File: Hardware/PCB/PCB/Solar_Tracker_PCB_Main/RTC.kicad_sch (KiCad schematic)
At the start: 1 part, among them IC4 PCF2131TFY

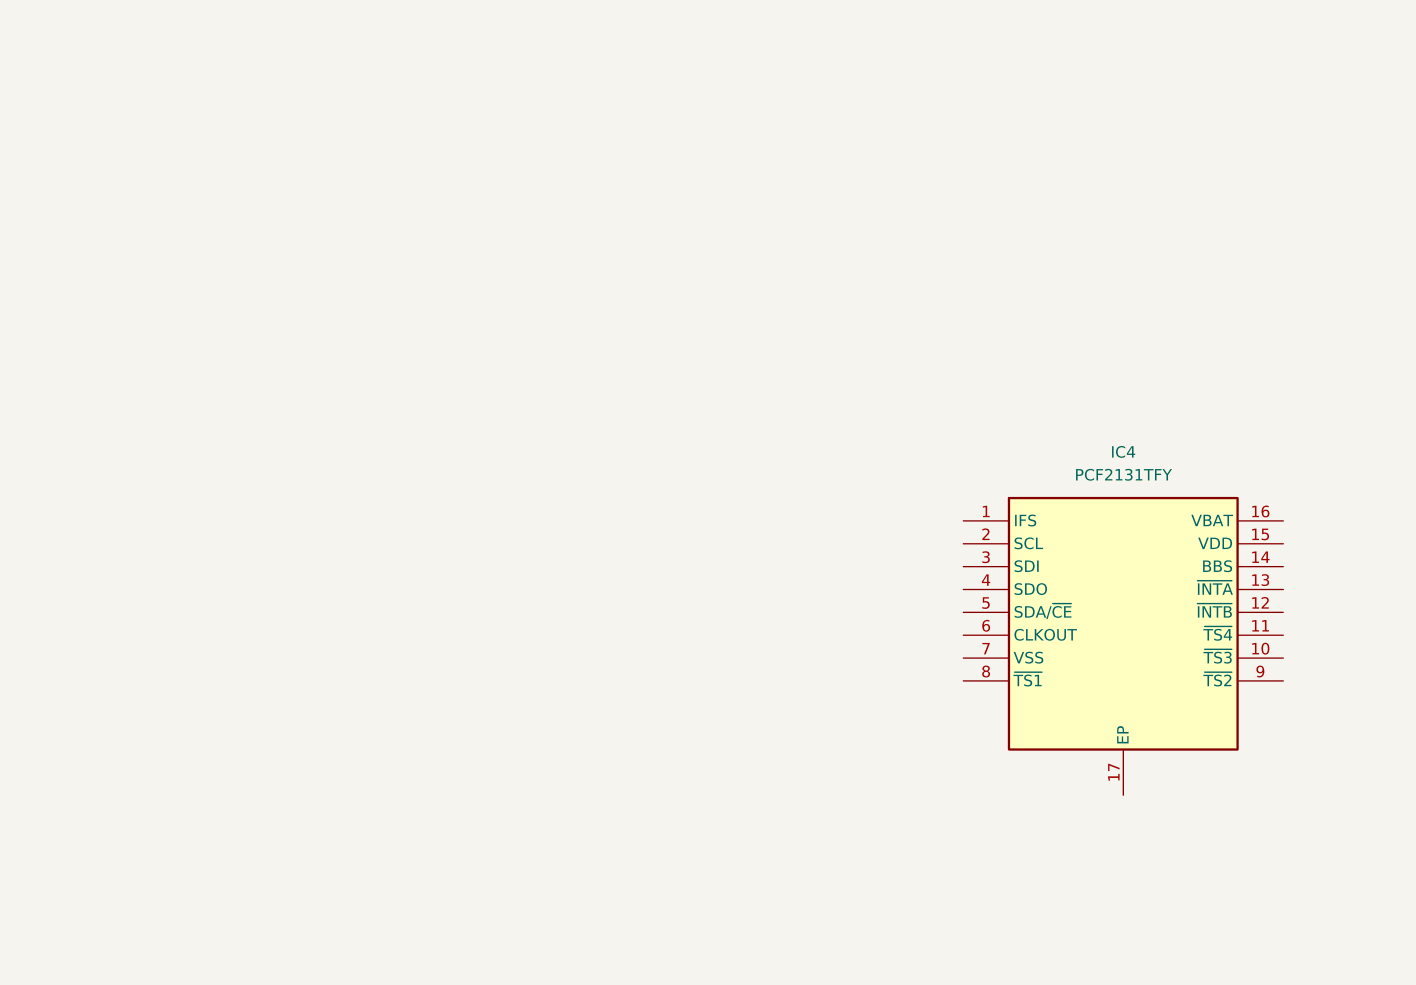
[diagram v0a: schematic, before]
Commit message: Actualizacion PCB Principal
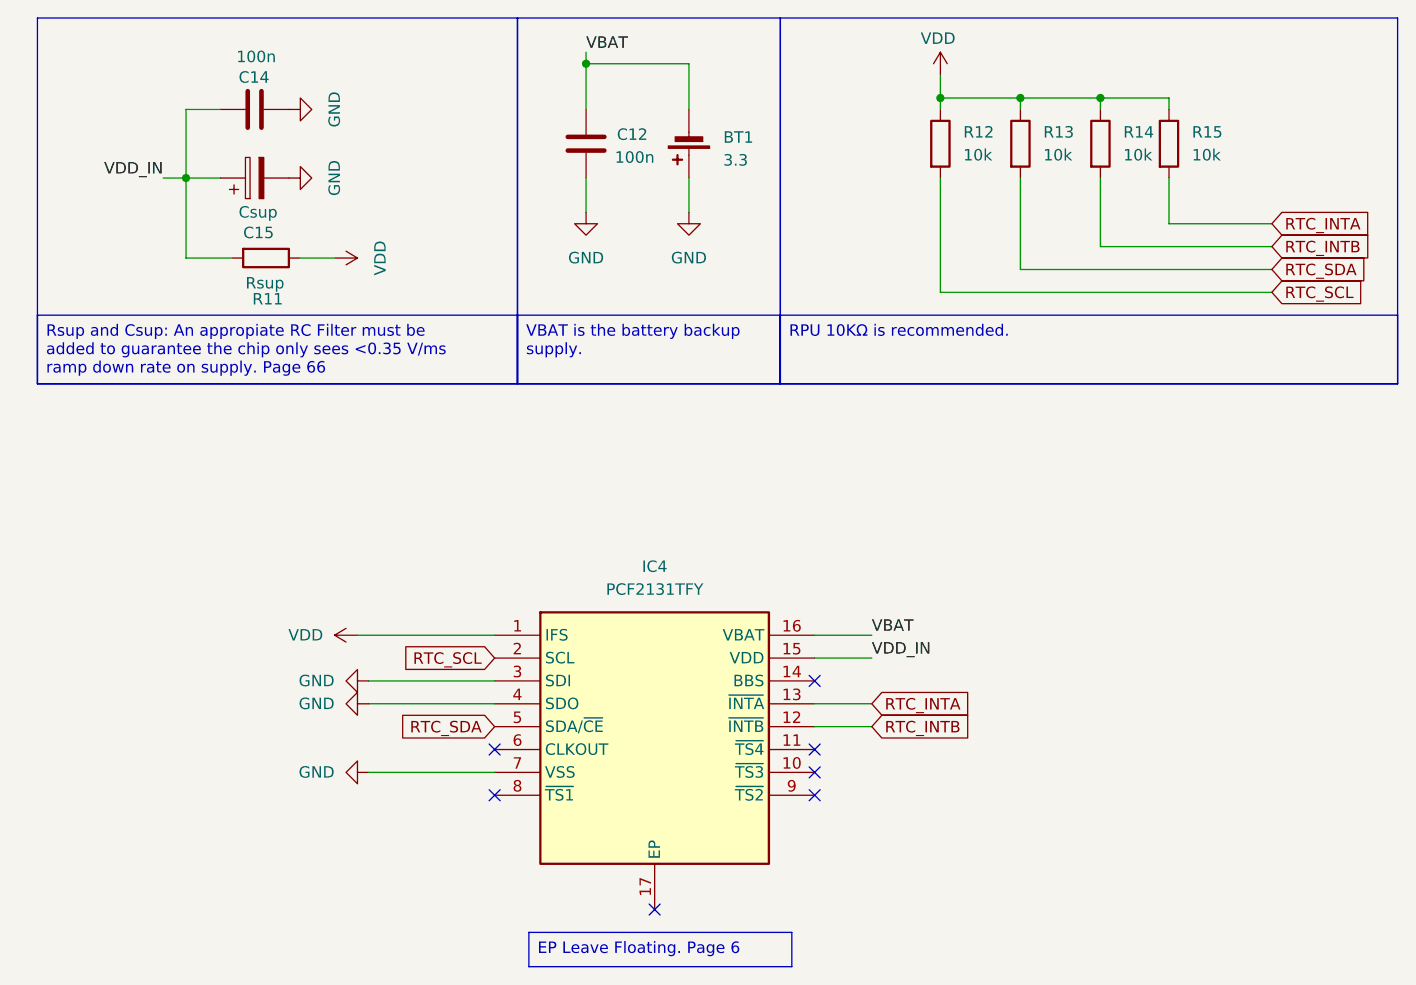
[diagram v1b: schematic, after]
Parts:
- added BT1: 3.3, symbol Device:Battery_Cell
- added C12, C14: 100n, symbol Device:C
- added C15: Csup, symbol Device:C_Polarized
- added R11: Rsup, symbol Device:R
- added R12, R13, R14, R15: 10k, symbol Device:R
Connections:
- net VDD: now reaches IC4.1 (IFS)
- net VDD: now also R11.1, R12.1, R13.1, R14.1, R15.1
- net RTC_INTB: now reaches IC4.12 (~{INTB})
- net RTC_INTB: now also R14.2
- net RTC_INTA: now reaches IC4.13 (~{INTA})
- net RTC_INTA: now also R15.2
- net VDD_IN: now reaches IC4.15 (VDD)
- net VDD_IN: now also C14.2, C15.1, R11.2
- net VBAT: now reaches IC4.16 (VBAT)
- net VBAT: now also BT1.2 (-), C12.2
- net RTC_SCL: now reaches IC4.2 (SCL)
- net RTC_SCL: now also R12.2
- net GND: now reaches IC4.3 (SDI)
- net GND: now also IC4.4 (SDO), IC4.7 (VSS), BT1.1 (+), C12.1, C14.1, C15.2
- net RTC_SDA: now reaches IC4.5 (SDA/~{CE})
- net RTC_SDA: now also R13.2
- no-connect marks 0 -> 7
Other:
- moved on the sheet: IC4

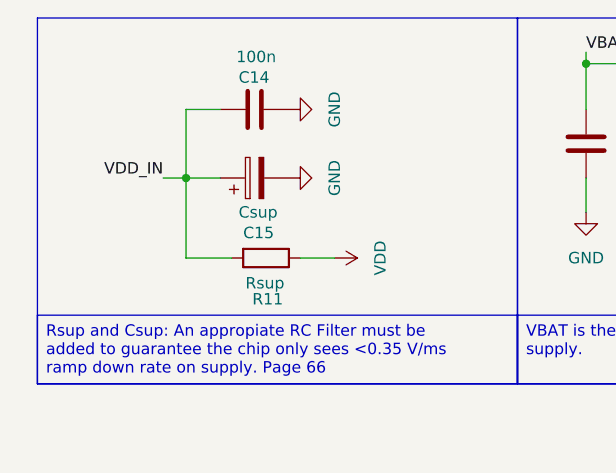
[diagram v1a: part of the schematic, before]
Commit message: actualizacion pcb principal
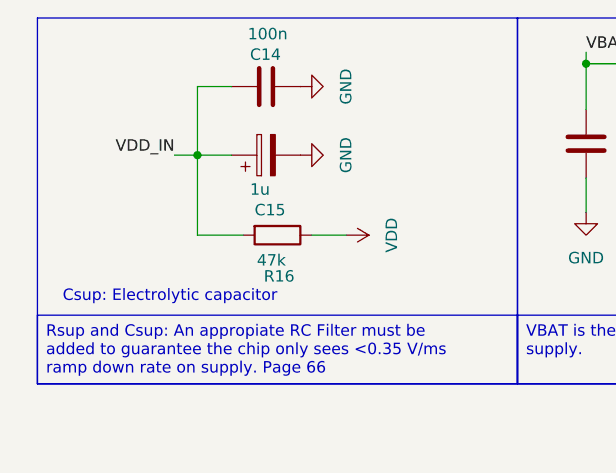
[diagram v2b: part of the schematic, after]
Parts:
- C15: value Csup -> 1u
- R16: renamed from R11; value Rsup -> 47k
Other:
- note added: "Csup: Electrolytic capacitor"
- moved on the sheet: C14, C15, R16
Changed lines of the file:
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@@
+		)
+	)
+	(text "Csup: Electrolytic capacitor"
+		(exclude_from_sim no)
+		(at 27.432 43.688 0)
+		(effects
+			(font
+				(size 1.27 1.27)
+			)
 		)
 	)
@@
 	)
 	(junction
-		(at 29.21 30.48)
+		(at 30.48 27.94)
 		(diameter 0)
 		(color 0 0 0 0)
@@
 	(wire
 		(pts
-			(xy 33.02 22.86) (xy 29.21 22.86)
-		)
-		(stroke
-			(width 0)
-			(type default)
-		)
-	)
-	(wire
-		(pts
-			(xy 34.29 39.37) (xy 29.21 39.37)
-		)
-		(stroke
-			(width 0)
-			(type default)
-		)
-	)
-	(wire
-		(pts
-			(xy 33.02 30.48) (xy 29.21 30.48)
+			(xy 34.29 20.32) (xy 30.48 20.32)
+		)
+		(stroke
+			(width 0)
+			(type default)
+		)
+	)
+	(wire
+		(pts
+			(xy 35.56 36.83) (xy 30.48 36.83)
+		)
+		(stroke
+			(width 0)
+			(type default)
+		)
+	)
+	(wire
+		(pts
+			(xy 34.29 27.94) (xy 30.48 27.94)
 		)
 		(stroke
@@
 	(wire
 		(pts
-			(xy 26.67 30.48) (xy 29.21 30.48)
+			(xy 27.94 27.94) (xy 30.48 27.94)
 		)
 		(stroke
@@
 	(wire
 		(pts
-			(xy 29.21 39.37) (xy 29.21 30.48)
+			(xy 30.48 36.83) (xy 30.48 27.94)
 		)
 		(stroke
@@
 	(wire
 		(pts
-			(xy 29.21 22.86) (xy 29.21 30.48)
+			(xy 30.48 20.32) (xy 30.48 27.94)
 		)
 		(stroke
@@
 	(wire
 		(pts
-			(xy 41.91 39.37) (xy 45.72 39.37)
+			(xy 43.18 36.83) (xy 46.99 36.83)
 		)
 		(stroke
@@
 	)
 	(label "VDD_IN"
-		(at 26.67 30.48 180)
+		(at 27.94 27.94 180)
 		(effects
 			(font
@@
 	(symbol
 		(lib_id "power:VDD")
-		(at 45.72 39.37 270)
+		(at 46.99 36.83 270)
 		(unit 1)
 		(exclude_from_sim no)
@@
 		(fields_autoplaced yes)
 		(property "Reference" "#PWR022"
-			(at 41.91 39.37 0)
+			(at 43.18 36.83 0)
 			(effects
 				(font
@@
 		)
 		(property "Value" "VDD"
-			(at 50.8 39.37 0)
+			(at 52.07 36.83 0)
 			(effects
 				(font
@@
 		)
 		(property "Footprint" ""
-			(at 45.72 39.37 0)
+			(at 46.99 36.83 0)
 			(effects
 				(font
@@
 		)
 		(property "Datasheet" ""
-			(at 45.72 39.37 0)
+			(at 46.99 36.83 0)
 			(effects
 				(font
@@
 		)
 		(property "Description" "Power symbol creates a global label with name \"VDD\""
-			(at 45.72 39.37 0)
+			(at 46.99 36.83 0)
 			(effects
 				(font
@@
 	(symbol
 		(lib_id "Device:R")
-		(at 38.1 39.37 270)
+		(at 39.37 36.83 270)
 		(unit 1)
 		(exclude_from_sim no)
@@
 		(on_board yes)
 		(dnp no)
-		(property "Reference" "R11"
-			(at 36.576 43.942 90)
+		(property "Reference" "R16"
+			(at 37.846 41.402 90)
 			(effects
 				(font
@@
 			)
 		)
-		(property "Value" "Rsup"
-			(at 35.814 42.164 90)
+		(property "Value" "47k"
+			(at 37.084 39.624 90)
 			(effects
 				(font
@@
 		)
 		(property "Footprint" ""
-			(at 38.1 37.592 90)
+			(at 39.37 35.052 90)
 			(effects
 				(font
@@
 		)
 		(property "Datasheet" "~"
-			(at 38.1 39.37 0)
+			(at 39.37 36.83 0)
 			(effects
 				(font
@@
 		)
 		(property "Description" "Resistor"
-			(at 38.1 39.37 0)
+			(at 39.37 36.83 0)
 			(effects
 				(font
@@
 			(project "Solar_Tracker_PCB_Main"
 				(path "/99b6ddd9-7ffe-4c85-972a-e0f594a166d4/f065d8bf-f34b-491d-8721-3ae145af2fae"
-					(reference "R11")
+					(reference "R16")
 					(unit 1)
 				)
@@
 	(symbol
 		(lib_id "Device:C_Polarized")
-		(at 36.83 30.48 90)
+		(at 38.1 27.94 90)
 		(unit 1)
 		(exclude_from_sim no)
@@
 		(dnp no)
 		(property "Reference" "C15"
-			(at 35.56 36.576 90)
+			(at 36.83 34.036 90)
 			(effects
 				(font
@@
 			)
 		)
-		(property "Value" "Csup"
-			(at 35.052 34.29 90)
+		(property "Value" "1u"
+			(at 36.322 31.75 90)
 			(effects
 				(font
@@
 		)
 		(property "Footprint" ""
-			(at 40.64 29.5148 0)
+			(at 41.91 26.9748 0)
 			(effects
 				(font
@@
 		)
 		(property "Datasheet" "~"
-			(at 36.83 30.48 0)
+			(at 38.1 27.94 0)
 			(effects
 				(font
@@
 		)
 		(property "Description" "Polarized capacitor"
-			(at 36.83 30.48 0)
+			(at 38.1 27.94 0)
 			(effects
 				(font
@@
 	(symbol
 		(lib_id "power:GND")
-		(at 40.64 30.48 90)
+		(at 41.91 27.94 90)
 		(unit 1)
 		(exclude_from_sim no)
@@
 		(fields_autoplaced yes)
 		(property "Reference" "#PWR024"
-			(at 46.99 30.48 0)
+			(at 48.26 27.94 0)
 			(effects
 				(font
@@
 		)
 		(property "Value" "GND"
-			(at 45.72 30.48 0)
+			(at 46.99 27.94 0)
 			(effects
 				(font
@@
 		)
 		(property "Footprint" ""
-			(at 40.64 30.48 0)
+			(at 41.91 27.94 0)
 			(effects
 				(font
@@
 		)
 		(property "Datasheet" ""
-			(at 40.64 30.48 0)
+			(at 41.91 27.94 0)
 			(effects
 				(font
@@
 		)
 		(property "Description" "Power symbol creates a global label with name \"GND\" , ground"
-			(at 40.64 30.48 0)
+			(at 41.91 27.94 0)
 			(effects
 				(font
@@
 	(symbol
 		(lib_id "Device:C")
-		(at 36.83 22.86 270)
+		(at 38.1 20.32 270)
 		(unit 1)
 		(exclude_from_sim no)
@@
 		(dnp no)
 		(property "Reference" "C14"
-			(at 35.052 19.304 90)
+			(at 36.322 16.764 90)
 			(effects
 				(font
@@
 		)
 		(property "Value" "100n"
-			(at 34.798 17.018 90)
+			(at 36.068 14.478 90)
 			(effects
 				(font
@@
 		)
 		(property "Footprint" ""
-			(at 33.02 23.8252 0)
+			(at 34.29 21.2852 0)
 			(effects
 				(font
@@
 		)
 		(property "Datasheet" "~"
-			(at 36.83 22.86 0)
+			(at 38.1 20.32 0)
 			(effects
 				(font
@@
 		)
 		(property "Description" "Unpolarized capacitor"
-			(at 36.83 22.86 0)
+			(at 38.1 20.32 0)
 			(effects
 				(font
@@
 	(symbol
 		(lib_id "power:GND")
-		(at 40.64 22.86 90)
+		(at 41.91 20.32 90)
 		(unit 1)
 		(exclude_from_sim no)
@@
 		(fields_autoplaced yes)
 		(property "Reference" "#PWR023"
-			(at 46.99 22.86 0)
+			(at 48.26 20.32 0)
 			(effects
 				(font
@@
 		)
 		(property "Value" "GND"
-			(at 45.72 22.86 0)
+			(at 46.99 20.32 0)
 			(effects
 				(font
@@
 		)
 		(property "Footprint" ""
-			(at 40.64 22.86 0)
+			(at 41.91 20.32 0)
 			(effects
 				(font
@@
 		)
 		(property "Datasheet" ""
-			(at 40.64 22.86 0)
+			(at 41.91 20.32 0)
 			(effects
 				(font
@@
 		)
 		(property "Description" "Power symbol creates a global label with name \"GND\" , ground"
-			(at 40.64 22.86 0)
-			(effects
-				(font
+			(at 41.91 20.32 0)
+			(effects
+				(font

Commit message: Actualizacion de Footprints Resistencias y Capacitores Main PCB
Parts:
- C12, C14, C15: footprint (none) -> Capacitor_SMD:C_0805_2012Metric_Pad1.18x1.45mm_HandSolder
- R12, R13, R14, R15, R16: footprint (none) -> Resistor_SMD:R_0805_2012Metric_Pad1.20x1.40mm_HandSolder
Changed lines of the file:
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@@
 			)
 		)
-		(property "Footprint" ""
+		(property "Footprint" "Resistor_SMD:R_0805_2012Metric_Pad1.20x1.40mm_HandSolder"
 			(at 111.252 26.67 90)
 			(effects
@@
 			)
 		)
-		(property "Footprint" ""
+		(property "Footprint" "Resistor_SMD:R_0805_2012Metric_Pad1.20x1.40mm_HandSolder"
 			(at 136.652 26.67 90)
 			(effects
@@
 			)
 		)
-		(property "Footprint" ""
+		(property "Footprint" "Resistor_SMD:R_0805_2012Metric_Pad1.20x1.40mm_HandSolder"
 			(at 129.032 26.67 90)
 			(effects
@@
 			)
 		)
-		(property "Footprint" ""
+		(property "Footprint" "Resistor_SMD:R_0805_2012Metric_Pad1.20x1.40mm_HandSolder"
 			(at 39.37 35.052 90)
 			(effects
@@
 			)
 		)
-		(property "Footprint" ""
+		(property "Footprint" "Capacitor_SMD:C_0805_2012Metric_Pad1.18x1.45mm_HandSolder"
 			(at 41.91 26.9748 0)
 			(effects
@@
 			)
 		)
-		(property "Footprint" ""
+		(property "Footprint" "Resistor_SMD:R_0805_2012Metric_Pad1.20x1.40mm_HandSolder"
 			(at 120.142 26.67 90)
 			(effects
@@
 			)
 		)
-		(property "Footprint" ""
+		(property "Footprint" "Capacitor_SMD:C_0805_2012Metric_Pad1.18x1.45mm_HandSolder"
 			(at 72.6948 22.86 0)
 			(effects
@@
 			)
 		)
-		(property "Footprint" ""
+		(property "Footprint" "Capacitor_SMD:C_0805_2012Metric_Pad1.18x1.45mm_HandSolder"
 			(at 34.29 21.2852 0)
 			(effects
